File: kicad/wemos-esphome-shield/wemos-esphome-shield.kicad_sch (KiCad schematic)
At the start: 18 parts, among them Q1 2N2219, Q2 2N2219, Q3 2N2219, T1 Transformer_1P_1S, U1 WeMos_D1_mini

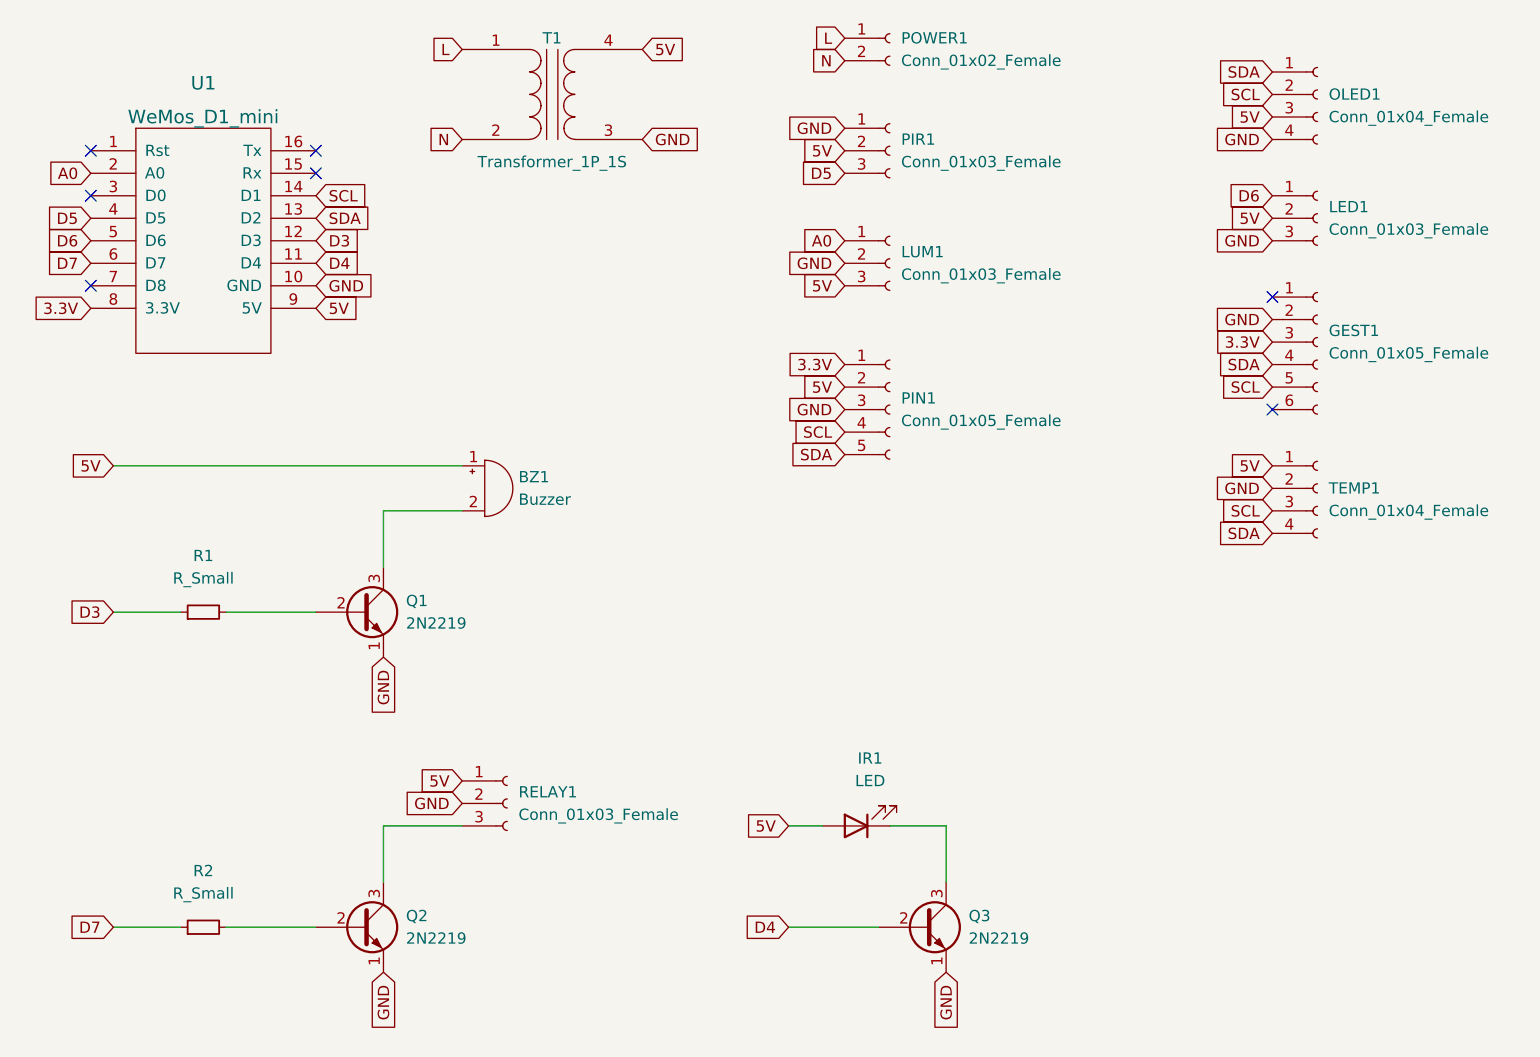
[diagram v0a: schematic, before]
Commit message: new footprints
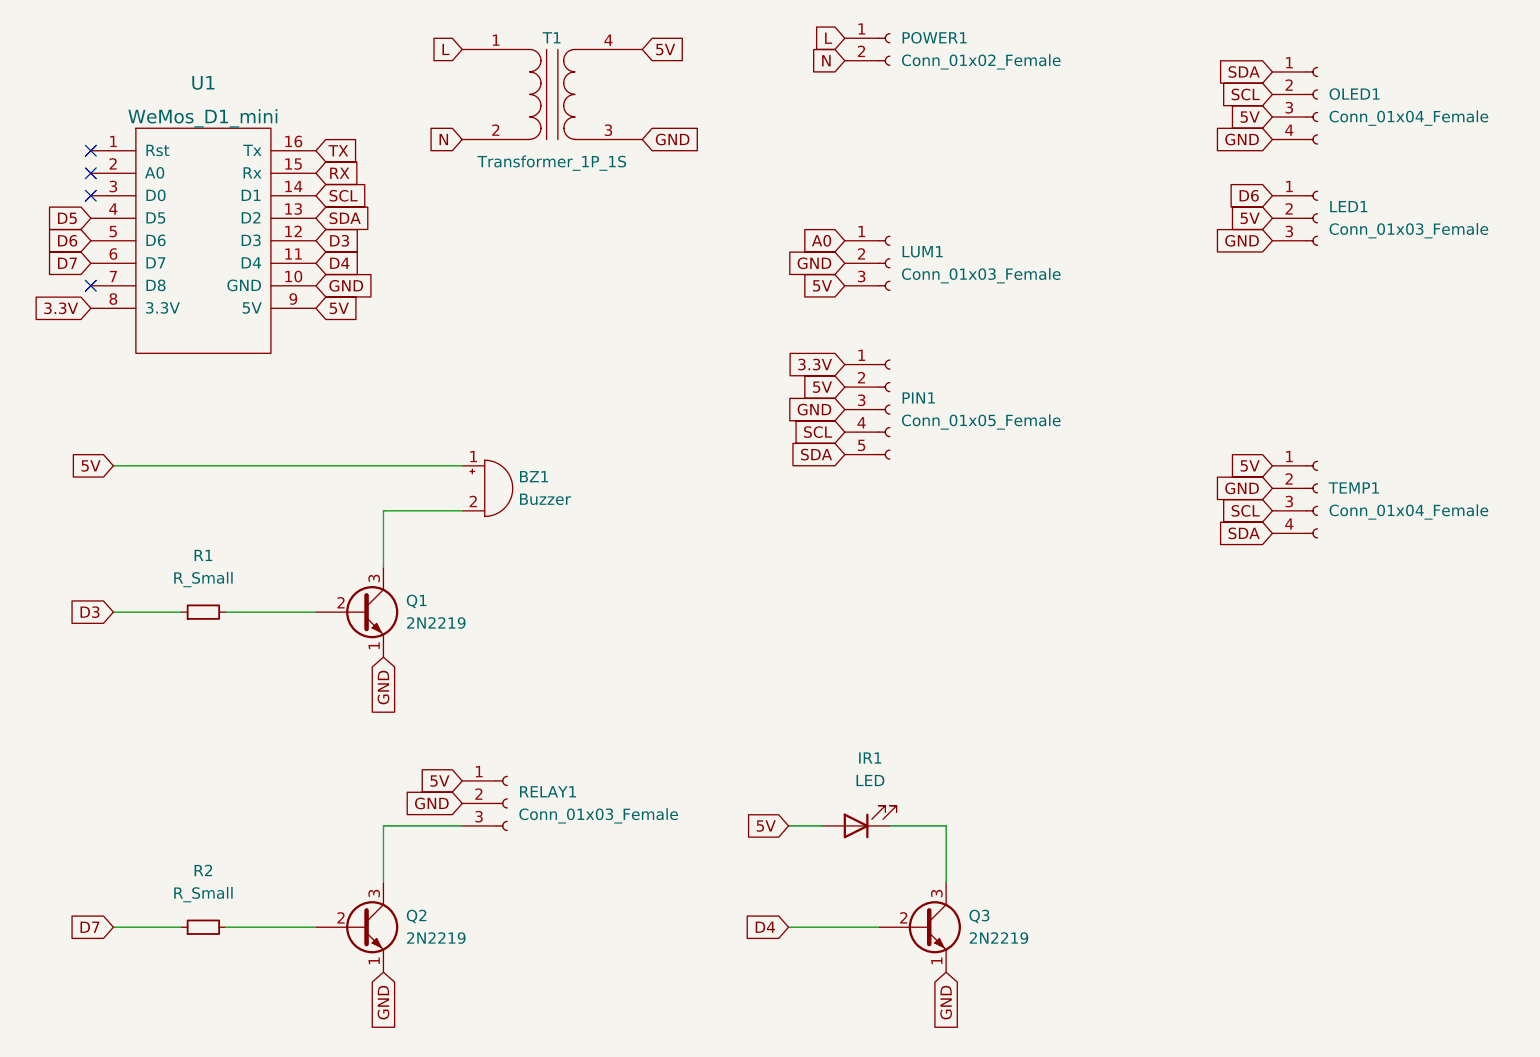
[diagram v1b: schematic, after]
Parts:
- removed GEST1: Conn_01x05_Female, internal:APDS9960, symbol Connector:Conn_01x06_Female
- removed PIR1: Conn_01x03_Female, internal:SR602, symbol Connector:Conn_01x03_Female
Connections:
- net A0: no longer U1.2 (A0)
- net RX: now reaches U1.15 (Rx)
- net TX: now reaches U1.16 (Tx)
- no-connect marks 7 -> 4
